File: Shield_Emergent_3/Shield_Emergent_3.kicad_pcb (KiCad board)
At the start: 2 copper layers, 28 x 36 mm, 17 parts, among them J1 USB3_B_Micro, J2 Conn_02x04_Odd_Even, J3 USB3_B_Micro, U3 SP3012-06UTG, U4 SP3012-06UTG, X1 USB_C_24pins

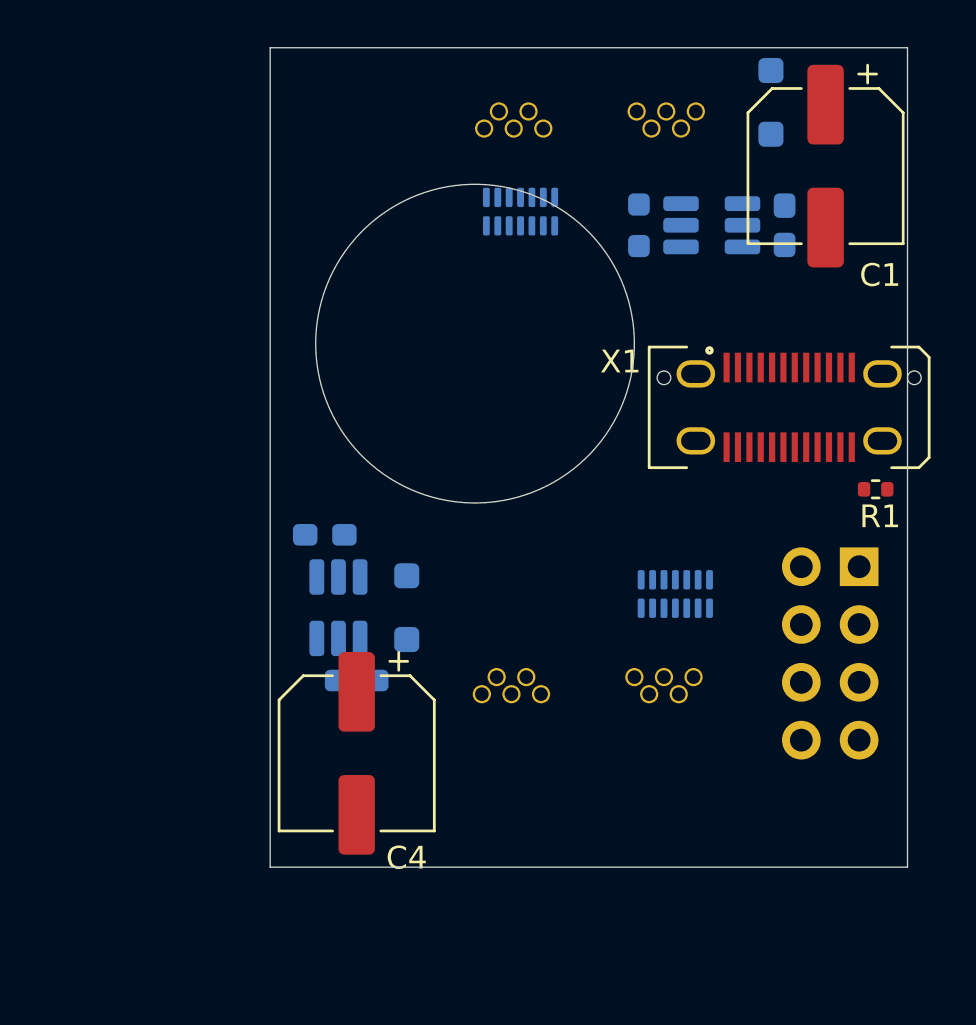
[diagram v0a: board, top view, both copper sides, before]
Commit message: v1.0 Geometry was modified
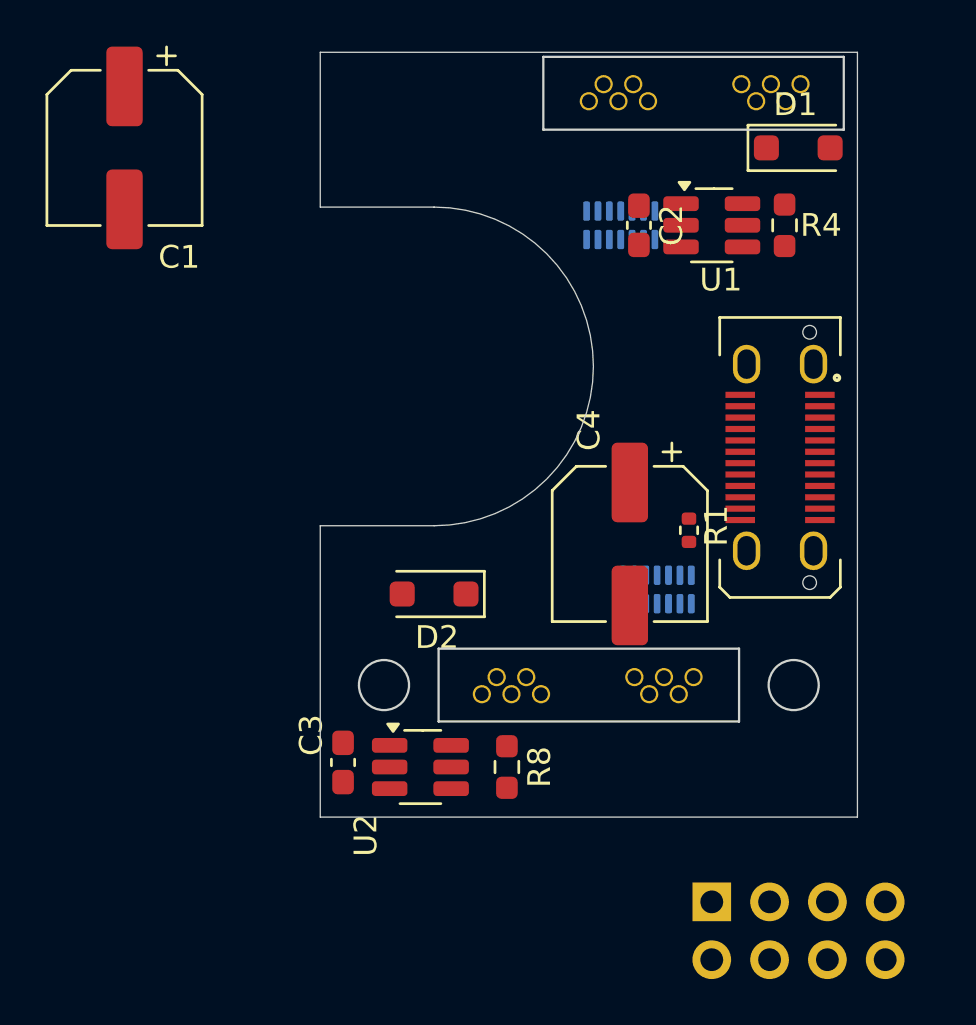
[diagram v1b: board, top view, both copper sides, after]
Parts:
- C2, C3, D1, D2, R4, R8, U1, U2: moved to F.Cu
- moved C1 30.8 mm to (-6.40, 4.40)
- moved J2 16.1 mm to (19.4, 37.5), turned to -90 degrees
- moved C4 15.1 mm to (15.8, 21.8)
- moved C3 10.0 mm to (3.20, 31.4), turned to -90 degrees
- moved R1 8.40 mm to (18.4, 21.2), turned to -90 degrees
- moved U2 7.87 mm to (6.60, 31.6), turned to 0 degrees
- moved R8 7.62 mm to (10.4, 31.6), turned to -90 degrees
- moved C2 6.40 mm to (16.2, 7.80)
- moved R4 6.40 mm to (22.6, 7.80)
- moved J1 4.75 mm to (23.3, 1.60)
- moved U3 4.44 mm to (15.4, 7.80)
- moved D1 2.33 mm to (23.2, 4.40), turned to 0 degrees
- moved X1 2.24 mm to (22.4, 18.0), turned to -90 degrees
- moved D2 1.34 mm to (7.20, 24.0), turned to 180 degrees
- moved U4 0.82 mm to (17.0, 23.8)
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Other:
- board size 28 x 36 mm -> 23.6 x 33.6 mm
